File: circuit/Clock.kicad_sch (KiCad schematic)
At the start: 12 parts, among them U1 WeMos_S2_mini

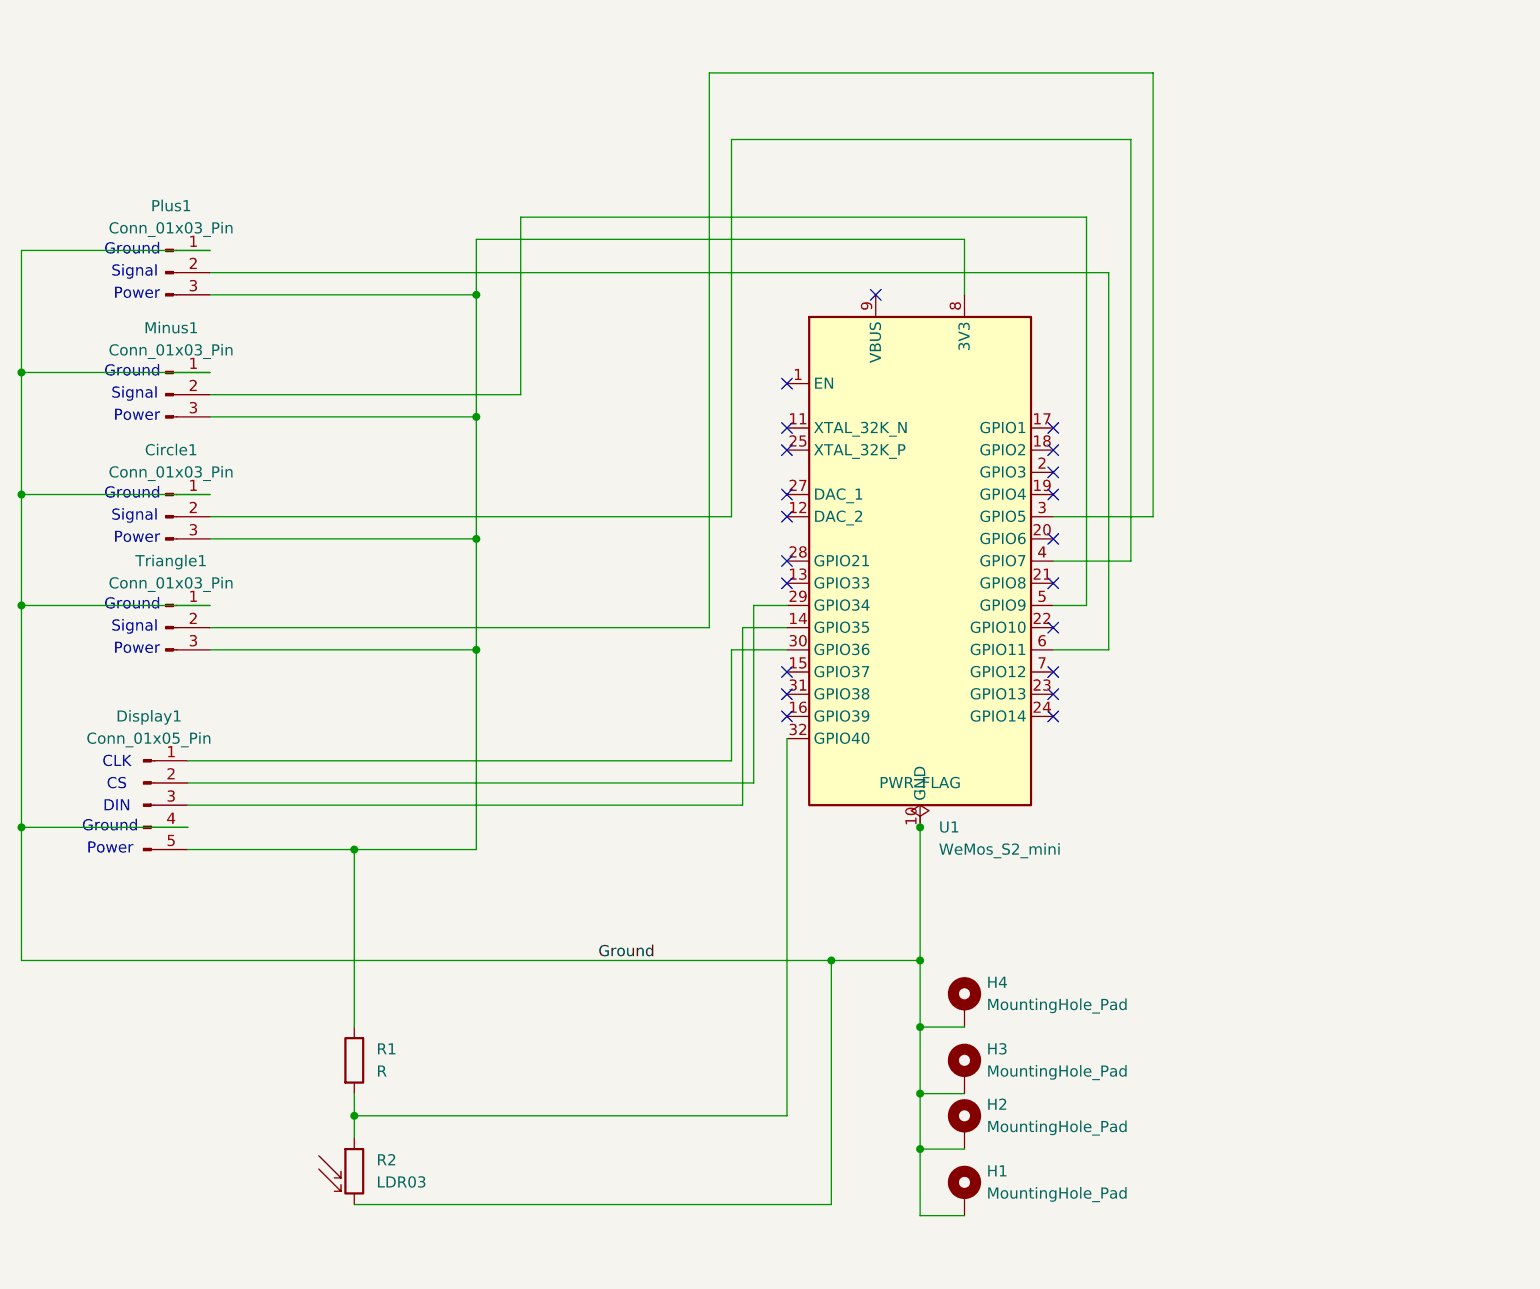
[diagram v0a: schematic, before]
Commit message: updated to be gooderer
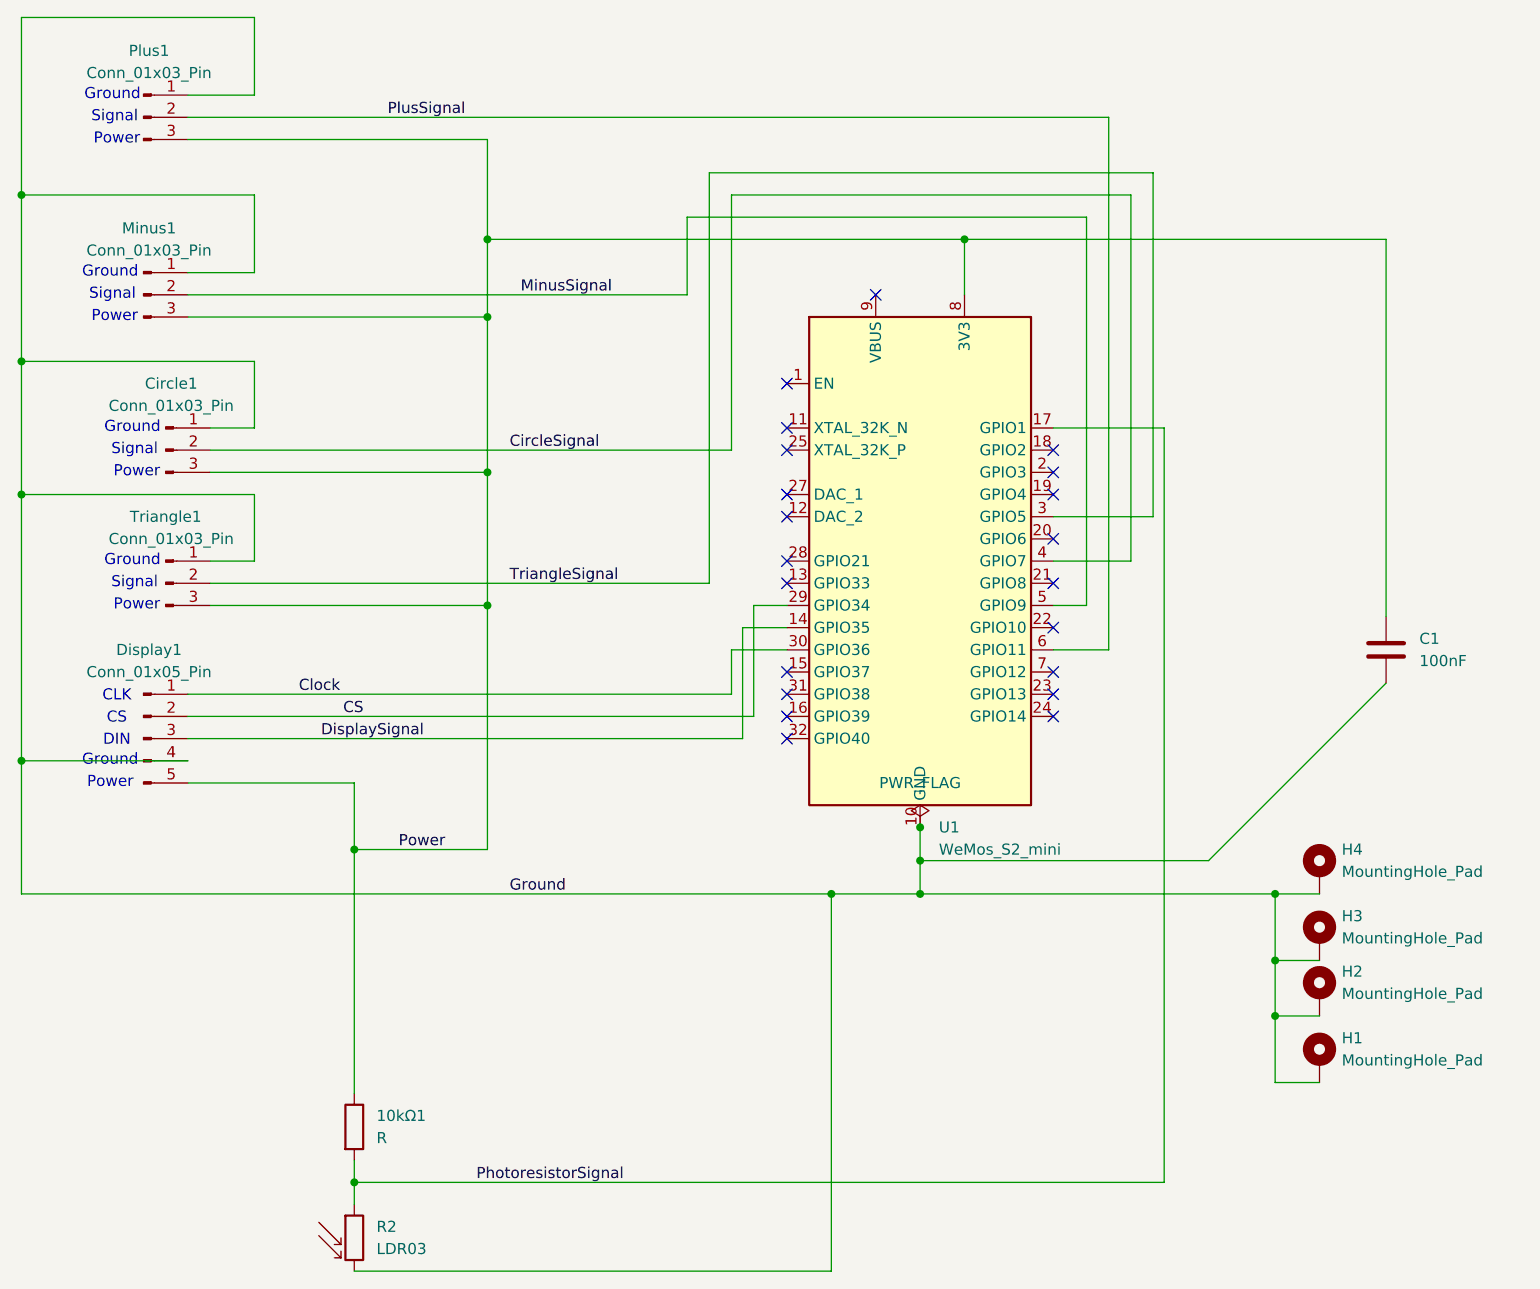
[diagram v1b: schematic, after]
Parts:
- added C1: 100nF, Capacitor_THT:C_Disc_D8.0mm_W2.5mm_P5.00mm, symbol Device:C
- renumbered R1 to 10kΩ1
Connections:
- net Ground: now also C1.2
- net MinusSignal: now reaches Minus1.2 (Pin_2), U1.5 (GPIO9)
- net Power: now reaches 10kΩ1.1, Circle1.3 (Pin_3), Display1.5 (Pin_5), Minus1.3 (Pin_3), Plus1.3 (Pin_3), Triangle1.3 (Pin_3), U1.8 (3V3)
- net Power: now also C1.1
- net DisplaySignal: now reaches Display1.3 (Pin_3), U1.14 (GPIO35)
- net PhotoresistorSignal: now reaches U1.17 (GPIO1)
- net PhotoresistorSignal: now also 10kΩ1.2, R2.1
- net CS: now reaches Display1.2 (Pin_2), U1.29 (GPIO34)
- net TriangleSignal: now reaches Triangle1.2 (Pin_2), U1.3 (GPIO5)
- net Clock: now reaches Display1.1 (Pin_1), U1.30 (GPIO36)
- net CircleSignal: now reaches Circle1.2 (Pin_2), U1.4 (GPIO7)
- net PlusSignal: now reaches Plus1.2 (Pin_2), U1.6 (GPIO11)
- now unconnected: U1.32 (GPIO40)
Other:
- moved on the sheet: 10kΩ1, Circle1, Display1, H1, H2, H3, H4, Minus1, Plus1, R2, Triangle1
